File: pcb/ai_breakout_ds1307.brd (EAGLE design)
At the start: 100 x 80 mm, 11 parts, among them J2 1X06, U1 DS1307SO8

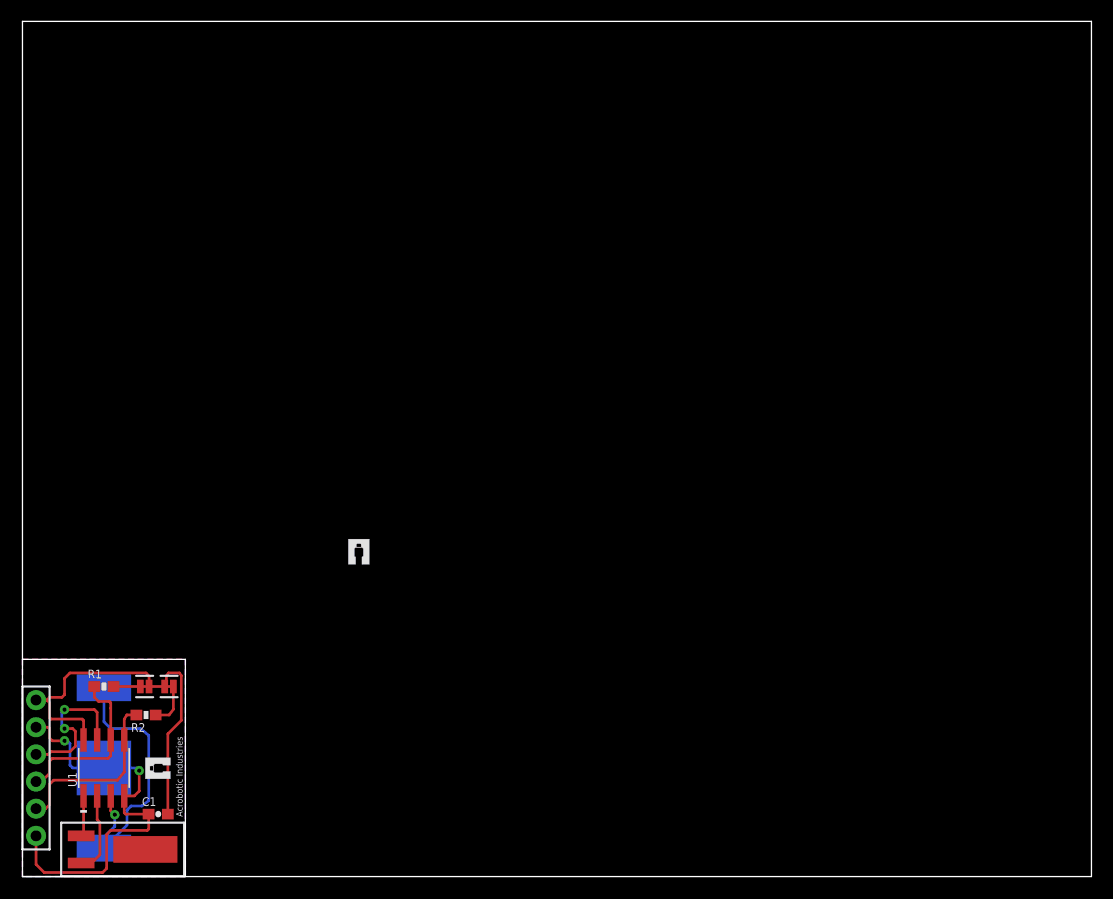
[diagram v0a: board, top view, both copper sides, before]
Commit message: board updated
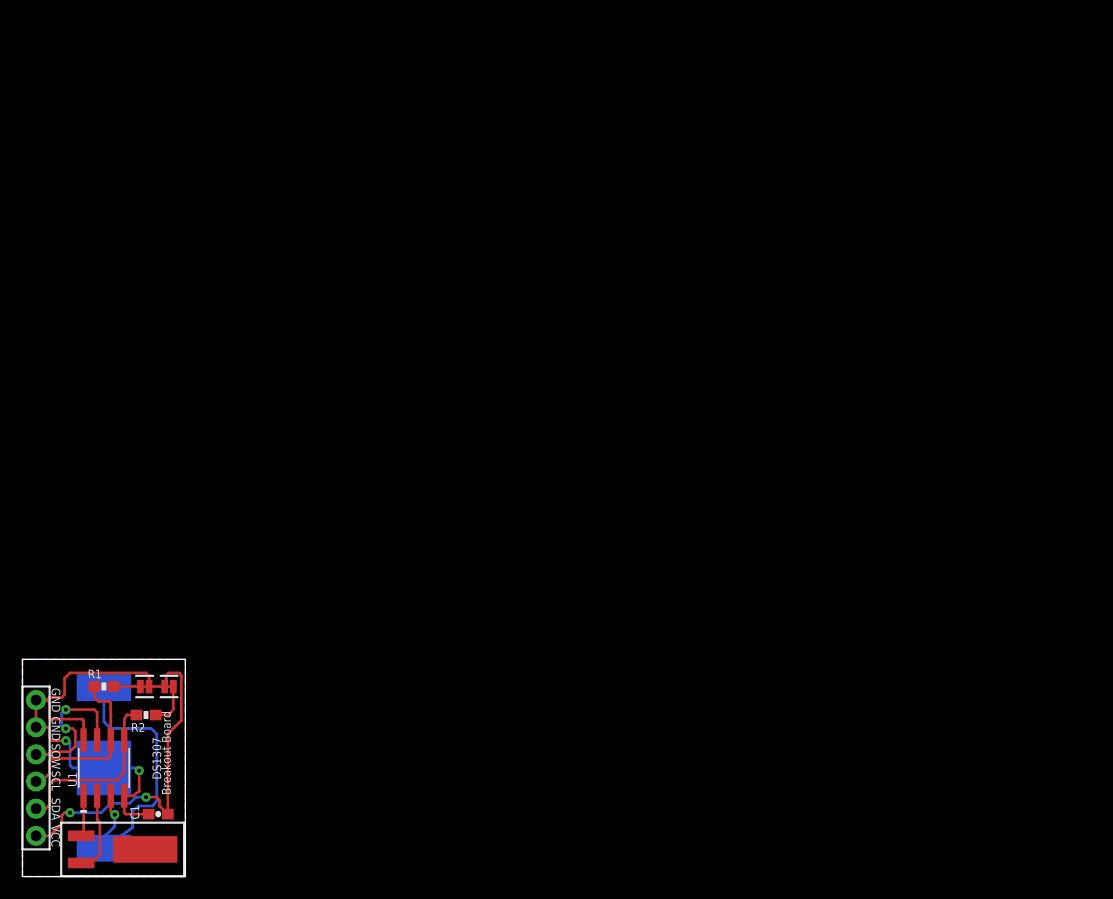
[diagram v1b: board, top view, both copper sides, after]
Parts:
- removed U$2: AI-LOGOXS, Ai_Miscellany:AI-LOGO-XS
- moved U$3 2.03 mm to (13.8, 11.2), flipped to the bottom, turned to 270 degrees
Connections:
- net GND: now also J2.6; no longer J2.1
- net VCC: now also J2.1; no longer J2.6
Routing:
- net GND: track 39.0 -> 23.1 mm
- net VCC: track 38.5 -> 52.7 mm, vias 0 -> 2
- net N$3: track 26.3 -> 27.8 mm
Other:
- board size 100 x 80 mm -> 15.2 x 20.3 mm
- board text added: "Breakout Board"
- board text added: "DS1307"
- board text added: "GND"
- board text added: "JCH V1.0"
- board text added: "SCL"
- board text added: "SDA"
- board text added: "SQW"
- board text added: "VCC"
- board text added: "www.acrobotic.com"
- board text removed: "Acrobotic Industries"
